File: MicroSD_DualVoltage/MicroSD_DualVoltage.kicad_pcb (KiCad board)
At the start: 2 copper layers, 25.4 x 26.7 mm, 21 parts, among them J1 Conn_01x08, U1 AP7365, U2 TXB0104PW

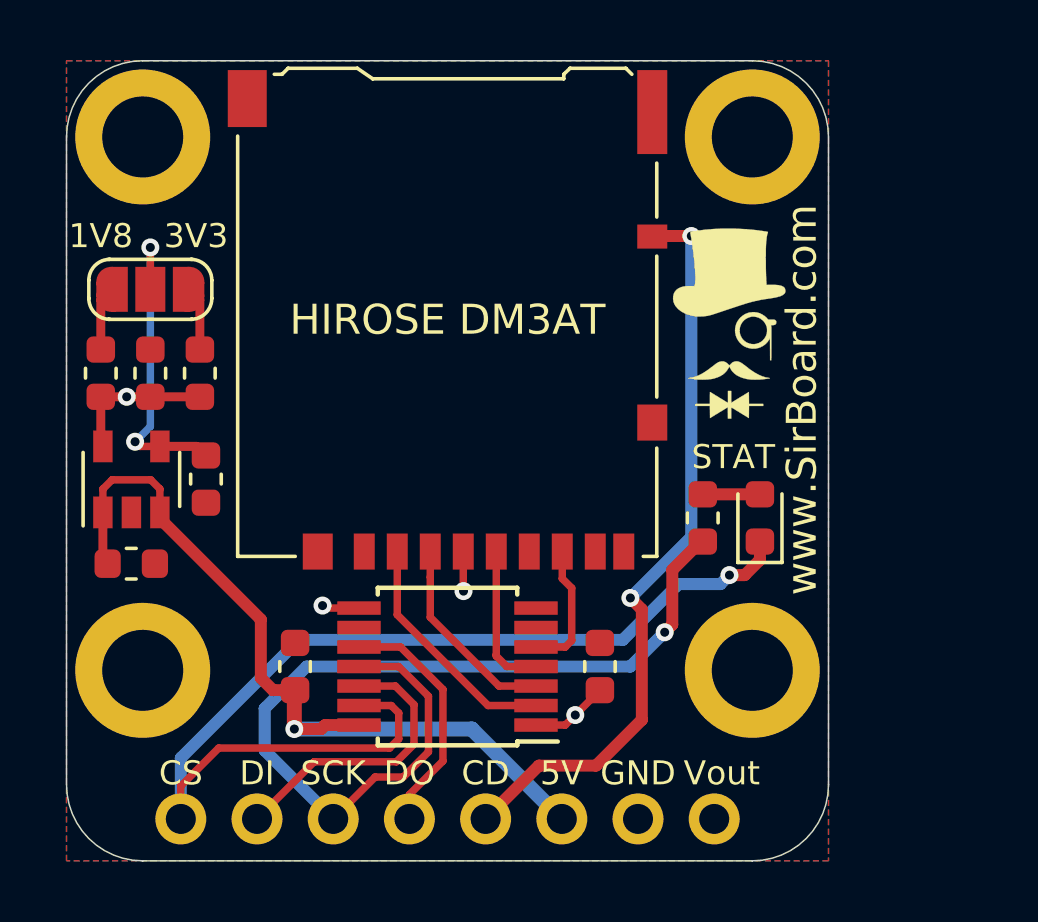
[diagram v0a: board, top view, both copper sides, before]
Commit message: Board Redesign
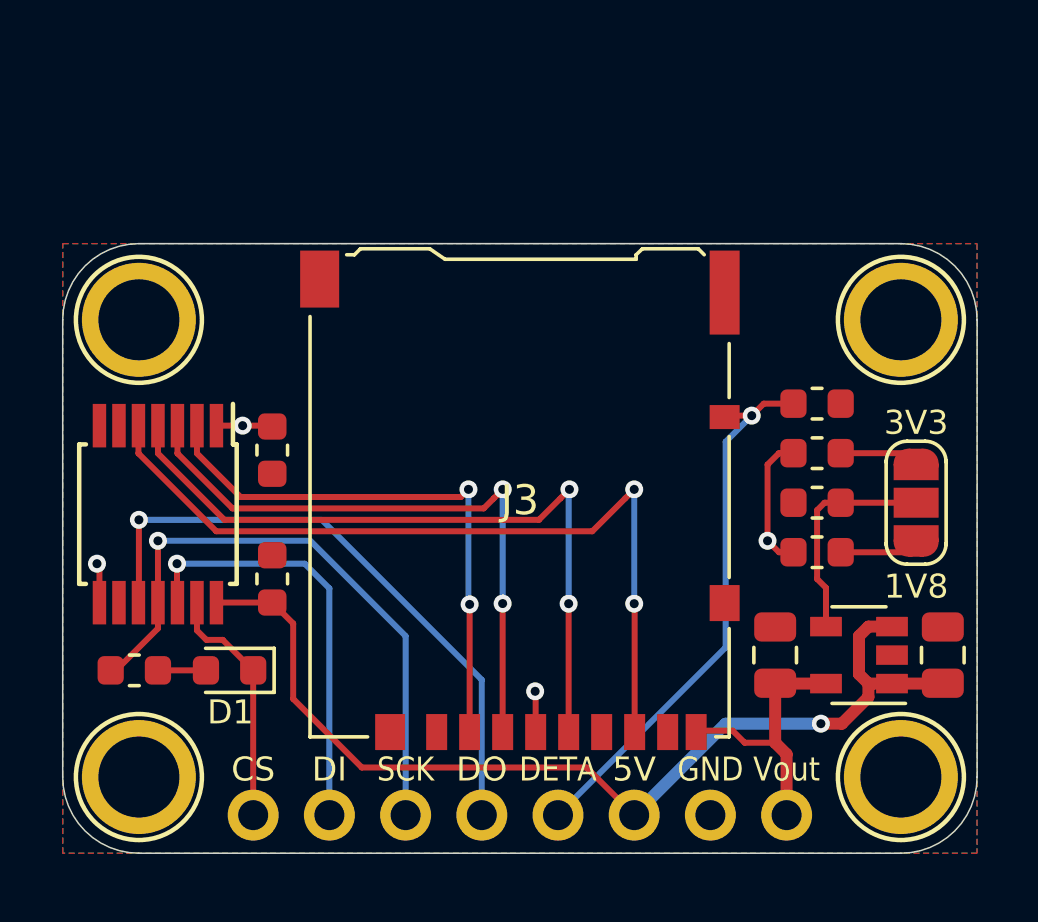
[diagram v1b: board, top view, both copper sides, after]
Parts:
- removed the G*** at (74.5, 28.2)
- removed the G*** at (65.2, 30.9)
- removed the G*** at (65.2, 39.5)
- added G***: LOGO, logo:SirBoard112x35, B.Cu at (67.4, 35.7)
- added G***: LOGO, logo:logo76x107, B.Cu at (67.4, 29.7)
- added R4: 10K, Resistor_SMD:R_0603_1608Metric, F.Cu at (77.5, 30.9)
- C1, C2: value 1uF -> 10uF; footprint Capacitor_SMD:C_0603_1608Metric -> Capacitor_SMD:C_0805_2012Metric
- H1, H2, H3, H4: footprint MountingHole:MountingHole_2.7mm_M2.5_ISO14580_Pad -> SirBoardLibrary:MountingHole_M2.5_SirBoard
- J3: renamed from HIROSE DM3AT
- R2: value 12K5 -> 12K4
- moved H3 29.6 mm to (54.9, 43.3), turned to 0 degrees
- moved H2 27.8 mm to (80.3, 28.1), turned to 0 degrees
- moved C1 27.2 mm to (81.7, 39.2), turned to 90 degrees
- moved JP1 26.5 mm to (80.8, 34.2), turned to 270 degrees
- moved U1 25.0 mm to (78.9, 39.2), turned to 180 degrees
- moved R2 24.6 mm to (77.5, 35.8), turned to 0 degrees
- moved C2 22.9 mm to (76.1, 39.2)
- moved R1 20.7 mm to (77.5, 32.5), turned to 0 degrees
- moved R3 20.4 mm to (77.5, 34.2), turned to 180 degrees
- moved R6 19.6 mm to (54.7, 39.8), turned to 0 degrees
- moved D1 18.4 mm to (57.9, 39.8), turned to 180 degrees
- moved C4 13.1 mm to (59.3, 32.4), turned to 270 degrees
- moved U2 10.9 mm to (55.5, 34.5), turned to 270 degrees
- moved J3 6.48 mm to (67.6, 34.1)
- moved H1 6.10 mm to (54.9, 28.1), turned to 0 degrees
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- renumbered STAT to D1
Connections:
- J3 pad 9: DETB -> VOUT
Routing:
- net CS: track 36.0 -> 8.18 mm, vias 1 -> 0
- net /DO_SD: track 4.38 -> 27.2 mm, vias 0 -> 2
- net /CLK_SD: track 4.95 -> 24.0 mm, vias 0 -> 2
- net /DI_SD: track 6.66 -> 20.8 mm, vias 0 -> 2
- net DO: track 8.16 -> 20.9 mm, vias 0 -> 1
- net /CS_SD: track 7.98 -> 18.7 mm, vias 0 -> 2
- net SCK: track 31.2 -> 20.6 mm
- net VOUT: track 10.1 -> 18.2 mm
- net DETA: track 25.0 -> 18.5 mm, vias 2 -> 1
- net VIN: track 27.4 -> 33.7 mm
- net DI: track 9.67 -> 14.3 mm, vias 0 -> 1
- net ADJ: track 10.6 -> 7.41 mm, vias 2 -> 0
- net Net-(JP1-Pad3): track 2.15 -> 2.66 mm
- net Net-(JP1-Pad1): track 2.15 -> 2.66 mm
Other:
- board size 25.4 x 26.7 mm -> 30.5 x 20.3 mm
- board text added: "DETA"
- board text added: "MicroSD to DIP Breakout With TXB0104 Level-Shift"
- board text removed: "CD"
- board text removed: "MicroSD Breakout TXB0104 Level Shift 1.8V AND 3.3V SD"
